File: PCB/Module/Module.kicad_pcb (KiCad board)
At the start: 2 copper layers, 30 x 30 mm, 22 parts, among them J1 SWD_Programmer, U1 PY32F002BF15P6TU, U2 PinHeaderTop, U3 PinHeaderRight, U4 PinHeaderBottom, U5 PinHeaderLeft, U6 Button

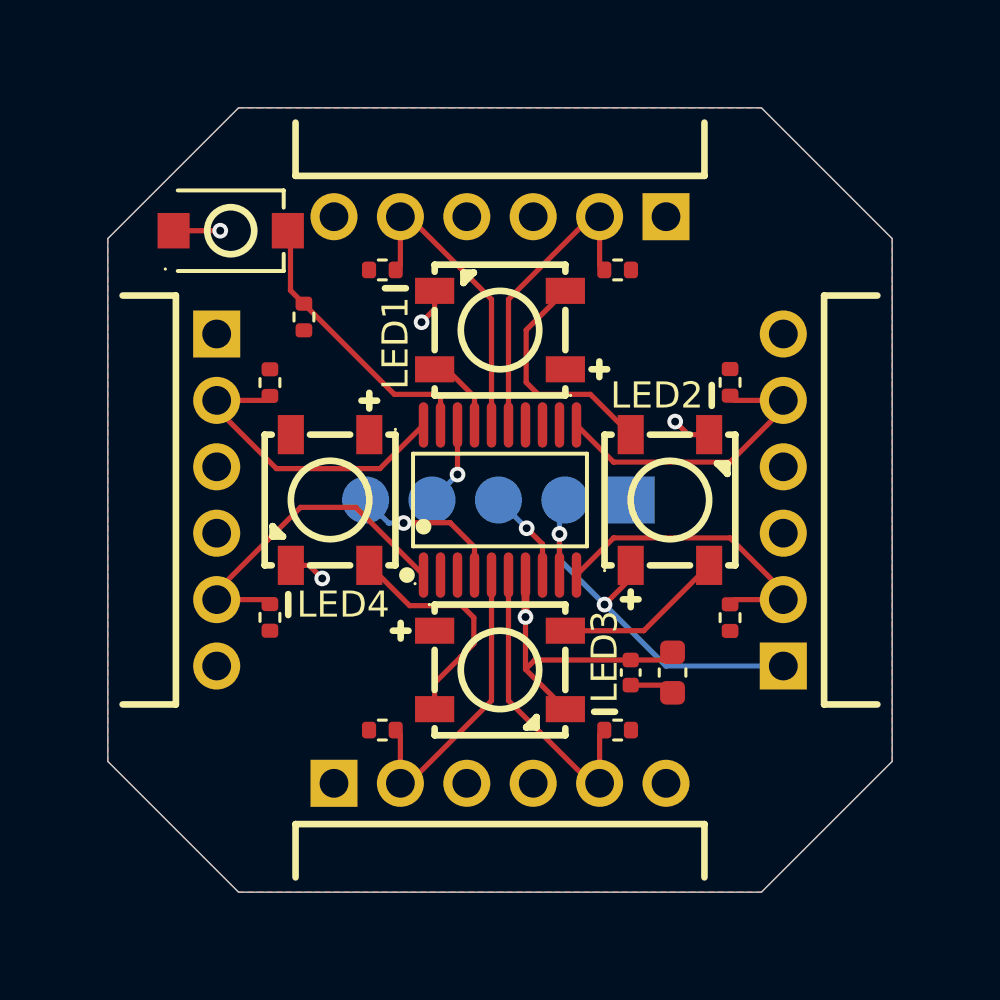
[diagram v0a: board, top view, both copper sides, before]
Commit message: Update PCB
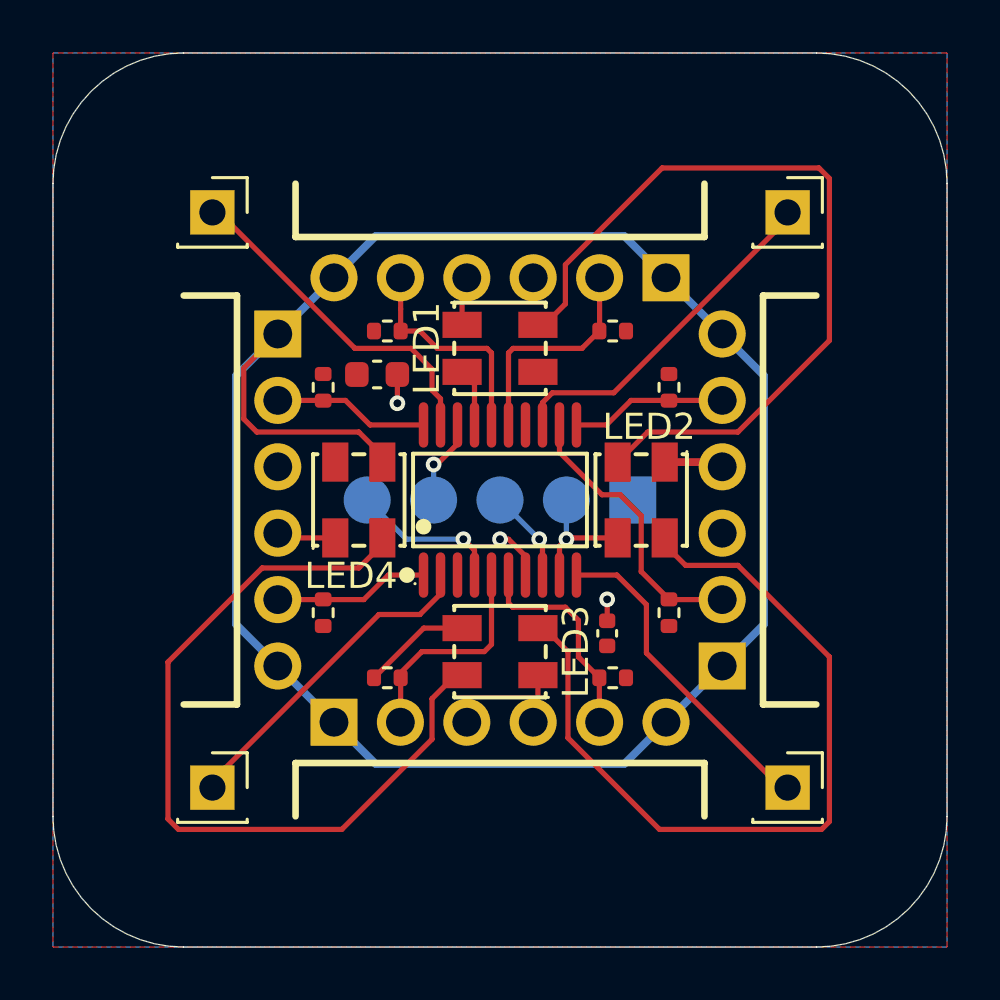
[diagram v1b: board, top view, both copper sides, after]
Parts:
- removed R9: 10k, Resistor_SMD:R_0402_1005Metric
- removed U6: Button, CustomFootprints:Button
- added J2: Shield_Connector_Top_Right, Connector_PinSocket_2.54mm:PinSocket_1x01_P2.54mm_Vertical, F.Cu at (161.0, 89.0)
- added J3: Shield_Connector_Bottom_Right, Connector_PinSocket_2.54mm:PinSocket_1x01_P2.54mm_Vertical, F.Cu at (161.0, 111.0)
- added J4: Shield_Connector_Top_Left, Connector_PinSocket_2.54mm:PinSocket_1x01_P2.54mm_Vertical, F.Cu at (139.0, 89.0)
- added J5: Shield_Connector_Bottom_Left, Connector_PinSocket_2.54mm:PinSocket_1x01_P2.54mm_Vertical, F.Cu at (139.0, 111.0)
- LED1, LED2, LED3, LED4: value LED-WS2812B -> SK6812MINI-HS; footprint CustomFootprints:LED-WS2812B -> CustomFootprints:LED-SK6812MINI-HS
- moved C1 16.1 mm to (145.3, 95.2), turned to 180 degrees
- moved R1 2.34 mm to (145.7, 93.5)
- moved R2 2.34 mm to (154.3, 93.5)
- moved R3 2.34 mm to (156.5, 95.7)
- moved R4 2.34 mm to (156.5, 104.3)
- moved U2 2.34 mm to (150.0, 91.5)
- moved U3 2.34 mm to (158.5, 100.0)
- moved U4 2.34 mm to (150.0, 108.5)
- moved U5 2.34 mm to (141.5, 100.0)
- moved R7 2.04 mm to (143.2, 104.3)
- moved R8 2.04 mm to (143.2, 95.7)
- moved R5 2.01 mm to (154.3, 106.8)
- moved R6 2.01 mm to (145.7, 106.8)
- moved C2 1.75 mm to (154.1, 105.1)
- moved LED2 1.10 mm to (155.4, 100.0), turned to 90 degrees
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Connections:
- LED1 pad 1: +5V -> GND
- LED1 pad 2: Net-(LED1-DOU) -> /LedIn
- LED1 pad 3: GND -> +5V
- LED1 pad 4: /LedIn -> Net-(LED1-DOUT)
- LED2 pad 1: +5V -> GND
- LED2 pad 2: Net-(LED2-DOU) -> Net-(LED1-DOUT)
- LED2 pad 3: GND -> +5V
- LED2 pad 4: Net-(LED1-DOU) -> Net-(LED2-DOUT)
- LED3 pad 1: +5V -> GND
- LED3 pad 2: Net-(LED3-DOU) -> Net-(LED2-DOUT)
- LED3 pad 3: GND -> +5V
- LED3 pad 4: Net-(LED2-DOU) -> Net-(LED3-DOUT)
- LED4 pad 1: +5V -> GND
- LED4 pad 2: unconnected-(LED4-DOU-Pad2) -> Net-(LED3-DOUT)
- LED4 pad 3: GND -> +5V
- LED4 pad 4: Net-(LED3-DOU) -> unconnected-(LED4-DOUT-Pad4)
- U1 pad 10: /DataRight1 -> /ShieldBottomRight
- U1 pad 12: unconnected-(U1-PB3-Pad12) -> /DataRight1
- U1 pad 13: unconnected-(U1-PB2-Pad13) -> /ShieldTopRight
- U1 pad 19: /ButtonRead -> /ShieldTopLeft
- U1 pad 2: unconnected-(U1-PA6-Pad2) -> /ShieldBottomLeft
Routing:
- net +5V: track 17.8 -> 87.3 mm, vias 2 -> 1
- net Net-(LED3-DOUT): track 0.00 -> 31.1 mm
- net Net-(LED2-DOUT): track 0.00 -> 31.0 mm
- net Net-(LED1-DOUT): track 0.00 -> 30.9 mm
- net /ShieldTopRight: track 0.00 -> 13.4 mm
- net /ShieldTopLeft: track 0.00 -> 13.1 mm
- net /ShieldBottomRight: track 0.00 -> 12.8 mm
- net /ShieldBottomLeft: track 0.00 -> 12.7 mm
- net /ButtonRead: track 10.7 -> 0.00 mm
- net Net-(LED1-DOU): track 8.95 -> 0.00 mm
- net Net-(LED3-DOU): track 8.95 -> 0.00 mm
- net GND: track 19.3 -> 12.2 mm, vias 5 -> 3
- net /DataLeft2: track 12.7 -> 5.96 mm
- net Net-(LED2-DOU): track 6.54 -> 0.00 mm
- net /DataLeft1: track 12.0 -> 5.96 mm
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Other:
- board size 30 x 30 mm -> 34.2 x 34.2 mm
- board text added: "+5V"
- board text added: "GND"
- board text added: "PCB"
- board text added: "Pogo Pins"
- board text added: "RST"
- board text added: "SWC"
- board text added: "SWD"
